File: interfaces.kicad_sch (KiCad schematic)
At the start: 38 parts, among them J16 Conn_02x12_Odd_Even, J3 Conn_01x15_Female, J4 Bus_M.2_Socket_E, Q1 BSS138APW, Q2 BSS138APW

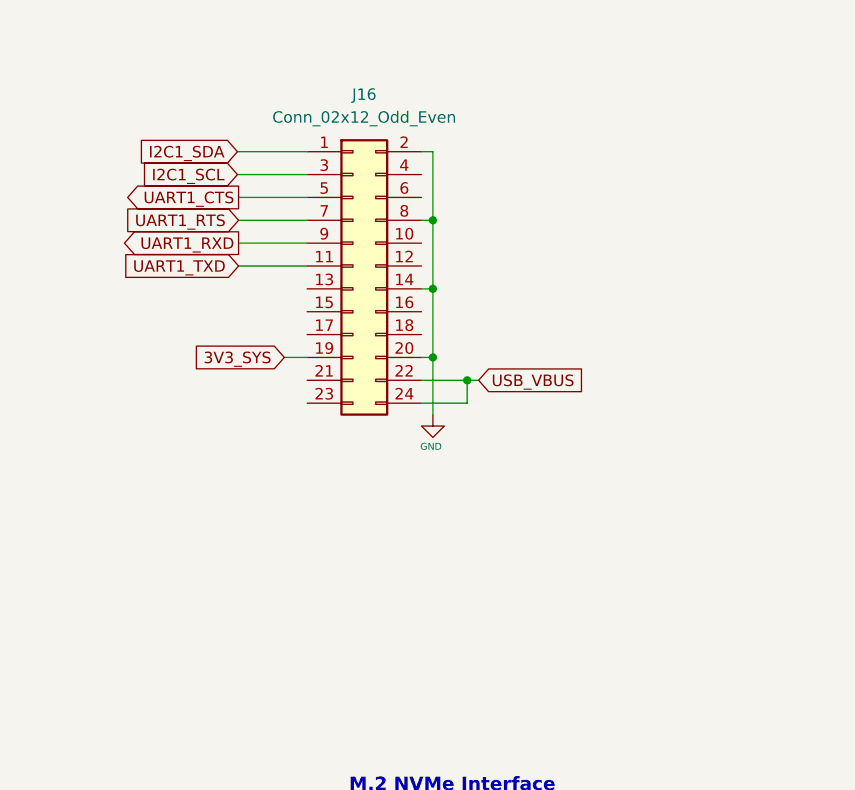
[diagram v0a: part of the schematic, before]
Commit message: Checkpoint
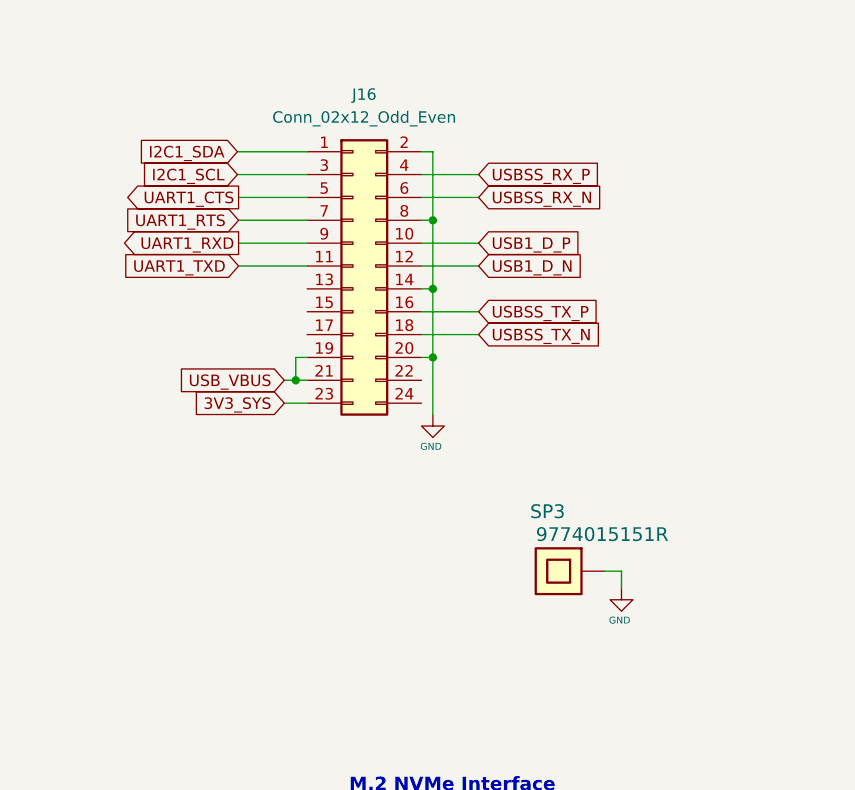
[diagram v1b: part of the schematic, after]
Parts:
- added SP3: 9774015151R, jetson-nano-baseboard-footprints:M2.5-2.5mm, symbol jetson-nano-baseboard:9774040151
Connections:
- net 3V3_SYS: now also J16.23 (Pin_23); no longer J16.19 (Pin_19)
- net GND: now also SP3.1
- net USB_VBUS: now also J16.19 (Pin_19), J16.21 (Pin_21); no longer J16.22 (Pin_22), J16.24 (Pin_24)
- net USB1_D_P: now reaches J16.10 (Pin_10)
- net USB1_D_N: now reaches J16.12 (Pin_12)
- net USBSS_TX_P: now reaches J16.16 (Pin_16)
- net USBSS_TX_N: now reaches J16.18 (Pin_18)
- net USBSS_RX_P: now reaches J16.4 (Pin_4)
- net USBSS_RX_N: now reaches J16.6 (Pin_6)
